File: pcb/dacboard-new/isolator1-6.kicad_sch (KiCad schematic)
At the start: 18 parts, among them U58 ISO6761FQDWRQ1, U83 ISO6761FQDWRQ1, U84 ISO6761FQDWRQ1, U85 ISO6761FQDWRQ1, U86 ISO6761FQDWRQ1, U87 ISO6761FQDWRQ1

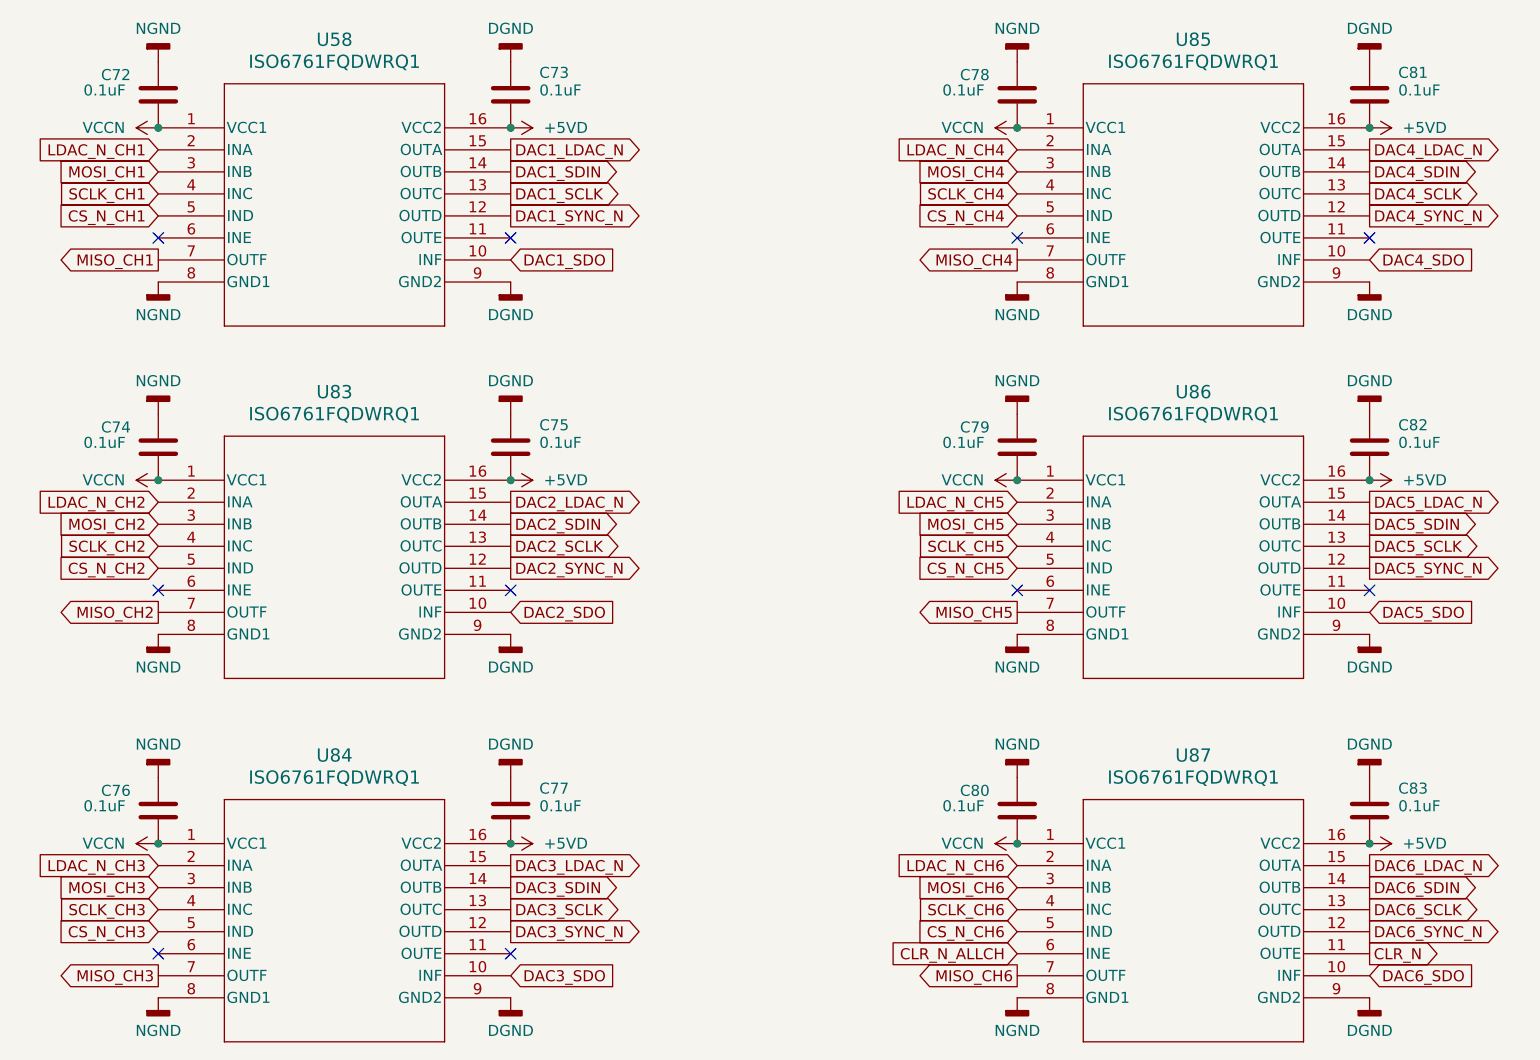
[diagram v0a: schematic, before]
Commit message: finished designing new pcb
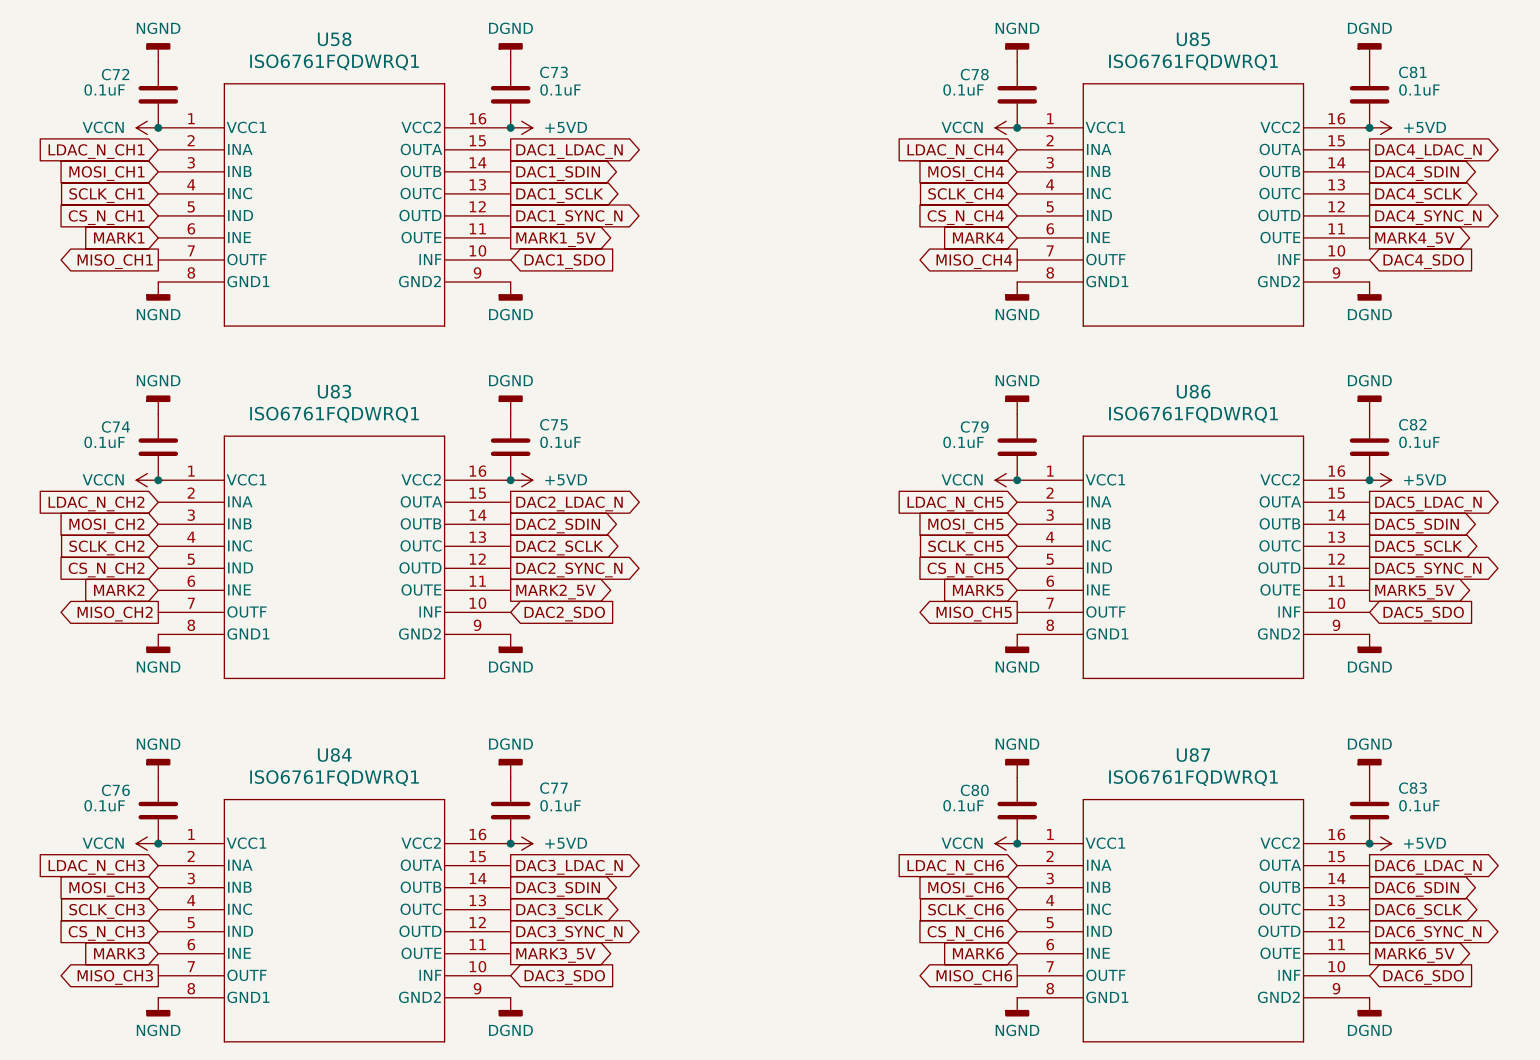
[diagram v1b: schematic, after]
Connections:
- net MARK2_5V: now reaches U83.11 (OUTE)
- net MARK2: now reaches U83.6 (INE)
- net MARK5_5V: now reaches U86.11 (OUTE)
- net MARK5: now reaches U86.6 (INE)
- net MARK3_5V: now reaches U84.11 (OUTE)
- net MARK3: now reaches U84.6 (INE)
- net MARK1_5V: now reaches U58.11 (OUTE)
- net MARK1: now reaches U58.6 (INE)
- net MARK4_5V: now reaches U85.11 (OUTE)
- net MARK4: now reaches U85.6 (INE)
- net CLR_N renamed MARK6_5V
- net CLR_N_ALLCH renamed MARK6
- no-connect marks 10 -> 0
